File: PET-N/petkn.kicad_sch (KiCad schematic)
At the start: 0 parts

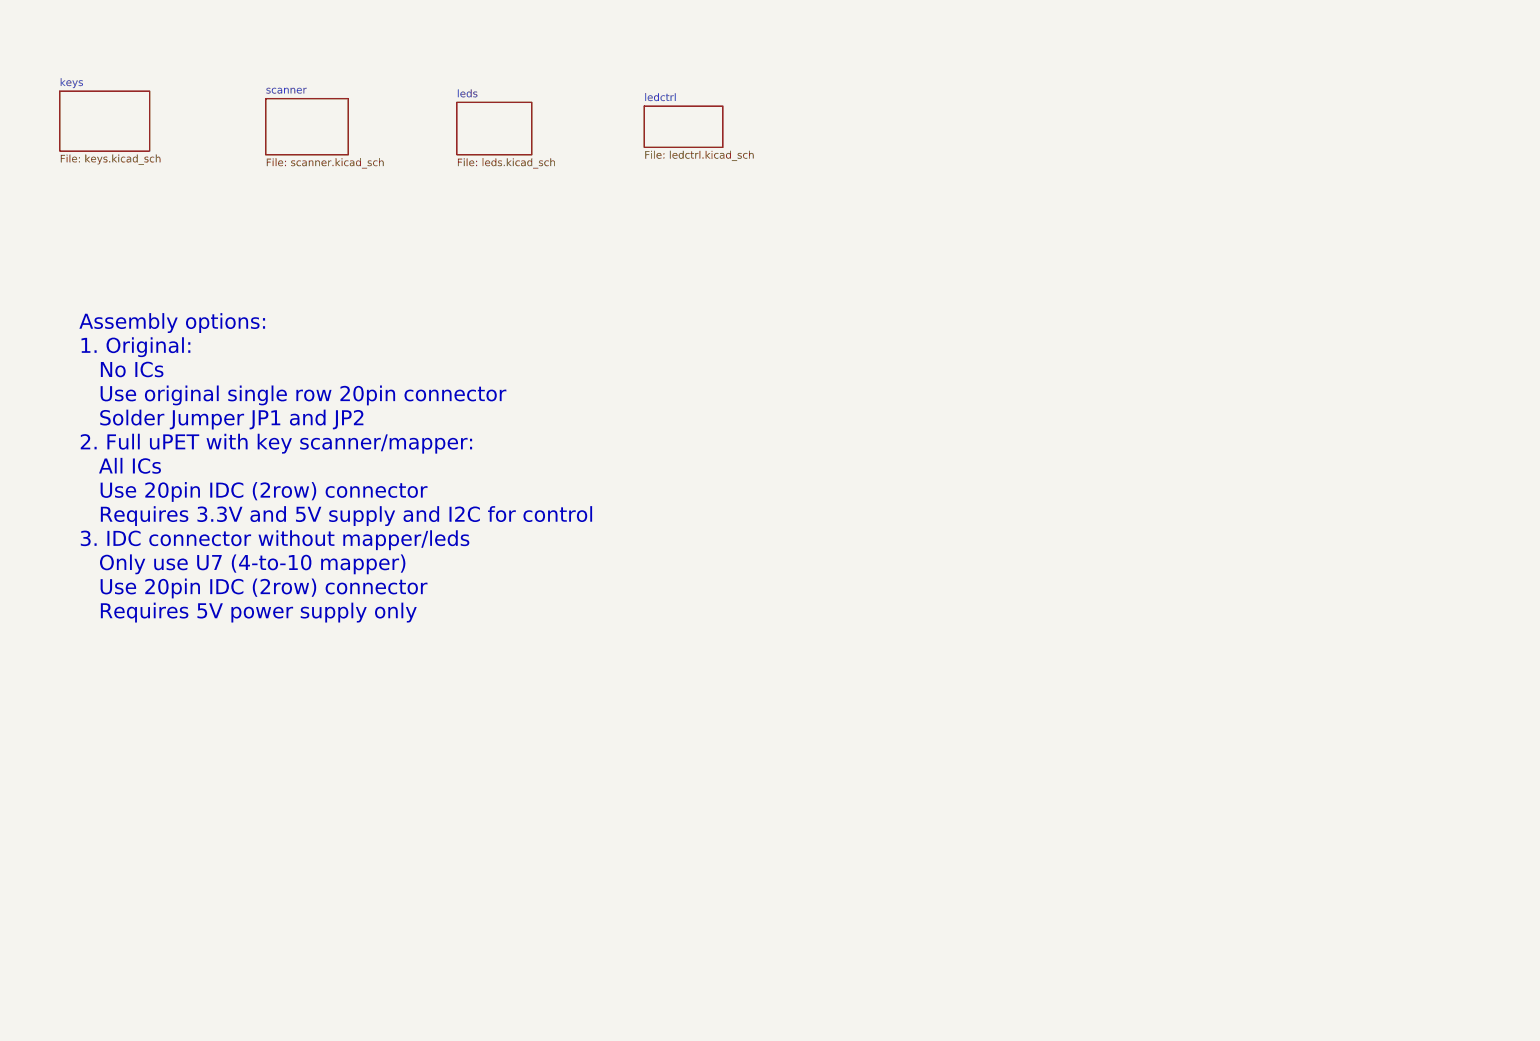
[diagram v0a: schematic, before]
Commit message: almost done routing; last checks still open
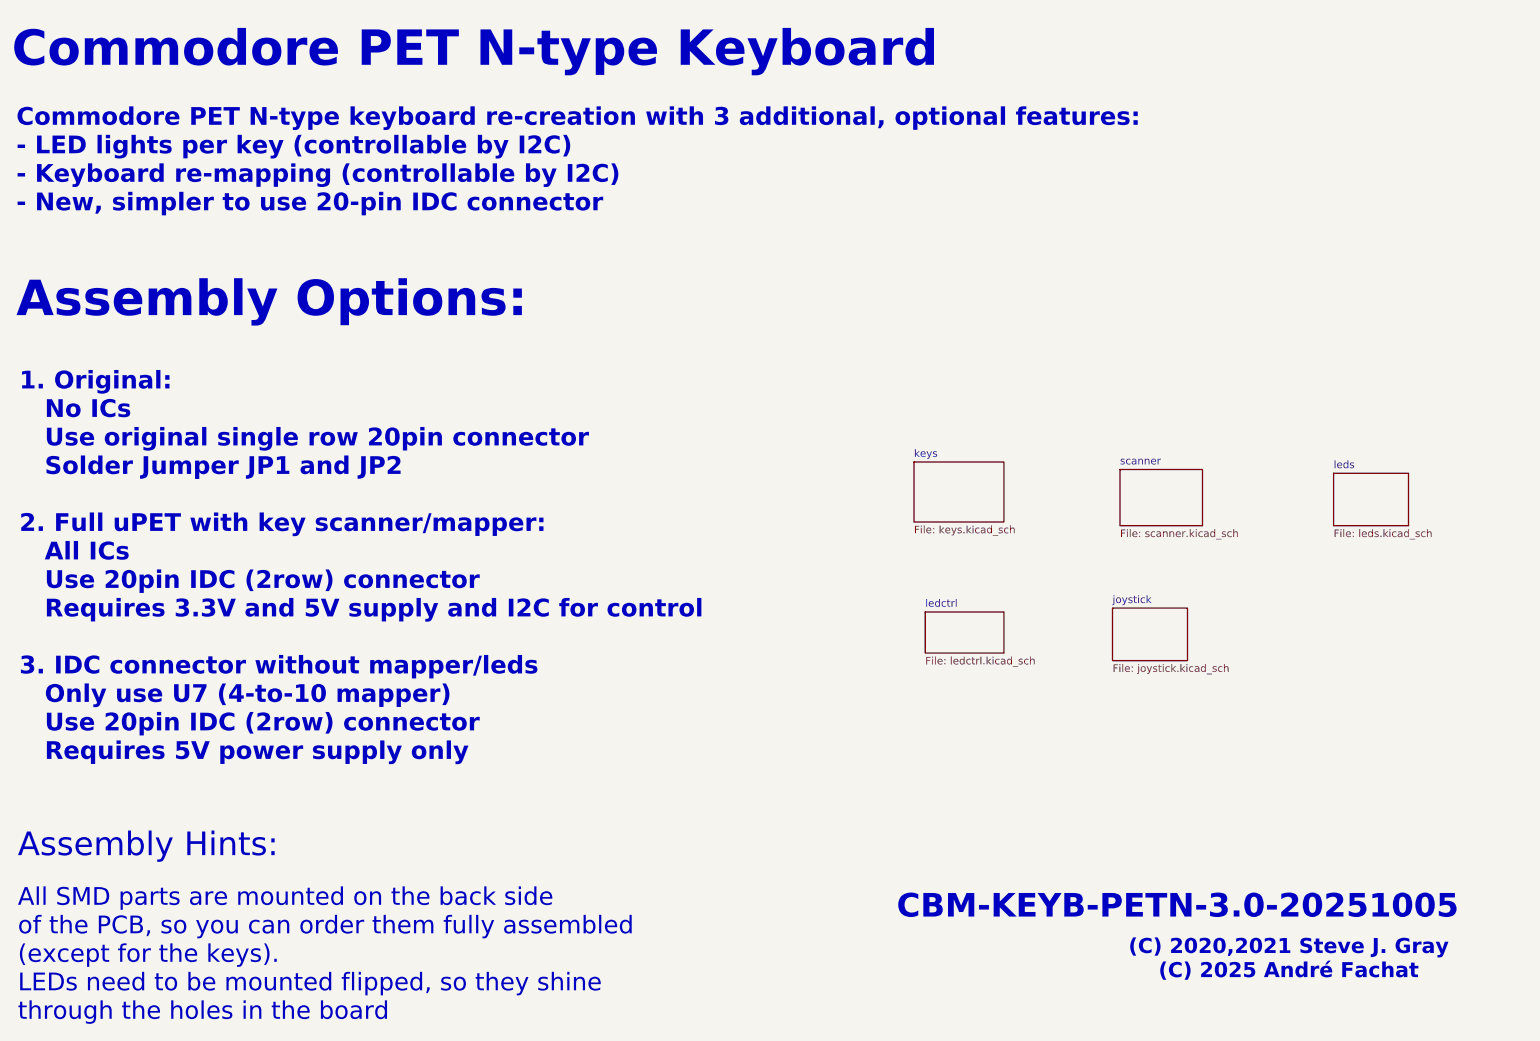
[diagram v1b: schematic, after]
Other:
- added sheet joystick (joystick.kicad_sch)
- note added: "(C) 2020,2021 Steve J. Gray (C) 2025 André Fachat"
- note added: "1. Original: No ICs Use original single row 20pin connector Solder Jumper JP1 and JP2 2. Full uPET with key scanner/mapper: All ICs Use 20pin IDC (2row) connector Requires 3.3V and 5V supply and I2C for control 3. IDC connector without mapper/leds Only use U7 (4-to-10 mapper) Use 20pin IDC (2row) connector Requires 5V power supply only"
- note added: "All SMD parts are mounted on the back side of the PCB, so you can order them fully assembled (except for the keys). LEDs need to be mounted flipped, so they shine through the holes in the board"
- note added: "Assembly Hints:"
- note added: "Assembly Options:"
- note added: "CBM-KEYB-PETN-3.0-20251005"
- note added: "Commodore PET N-type Keyboard"
- note added: "Commodore PET N-type keyboard re-creation with 3 additional, optional features: - LED lights per key (controllable by I2C) - Keyboard re-mapping (controllable by I2C) - New, simpler to use 20-pin IDC connector"
- note removed: "Assembly options: 1. Original: No ICs Use original single row 20pin connector Solder Jumper JP1 and JP2 2. Full uPET with key scanner/mapper: All ICs Use 20pin IDC (2row) connector Requires 3.3V and 5V supply and I2C for control 3. IDC connector without mapper/leds Only use U7 (4-to-10 mapper) Use 20pin IDC (2row) connector Requires 5V power supply only"
- company: Steve J. Gray -> Steve J. Gray, André Fachat
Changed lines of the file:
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@@
 	(title_block
 		(title "PET/CBM \"N\" Keyboard")
-		(date "2020-12-18")
-		(rev "N-V1-R1")
-		(company "Steve J. Gray")
-	)
-	(text "Assembly options:\n1. Original:\n   No ICs\n   Use original single row 20pin connector\n   Solder Jumper JP1 and JP2\n2. Full uPET with key scanner/mapper:\n   All ICs\n   Use 20pin IDC (2row) connector\n   Requires 3.3V and 5V supply and I2C for control\n3. IDC connector without mapper/leds\n   Only use U7 (4-to-10 mapper)\n   Use 20pin IDC (2row) connector\n   Requires 5V power supply only"
-		(exclude_from_sim no)
-		(at 43.942 98.806 0)
+		(date "2025-10-05")
+		(rev "N-V3-R0")
+		(company "Steve J. Gray, André Fachat")
+	)
+	(text "1. Original:\n   No ICs\n   Use original single row 20pin connector\n   Solder Jumper JP1 and JP2\n\n2. Full uPET with key scanner/mapper:\n   All ICs\n   Use 20pin IDC (2row) connector\n   Requires 3.3V and 5V supply and I2C for control\n\n3. IDC connector without mapper/leds\n   Only use U7 (4-to-10 mapper)\n   Use 20pin IDC (2row) connector\n   Requires 5V power supply only"
+		(exclude_from_sim no)
+		(at 33.782 115.57 0)
+		(effects
+			(font
+				(size 3 3)
+				(thickness 0.6)
+				(bold yes)
+			)
+			(justify left)
+		)
+	)
+	(text "All SMD parts are mounted on the back side\nof the PCB, so you can order them fully assembled\n(except for the keys).\nLEDs need to be mounted flipped, so they shine\nthrough the holes in the board"
+		(exclude_from_sim no)
+		(at 33.528 181.356 0)
+		(effects
+			(font
+				(size 3 3)
+				(thickness 0.375)
+			)
+			(justify left)
+		)
+	)
+	(text "Commodore PET N-type keyboard re-creation with 3 additional, optional features:\n- LED lights per key (controllable by I2C)\n- Keyboard re-mapping (controllable by I2C)\n- New, simpler to use 20-pin IDC connector"
+		(exclude_from_sim no)
+		(at 33.274 46.736 0)
+		(effects
+			(font
+				(size 3 3)
+				(thickness 0.6)
+				(bold yes)
+			)
+			(justify left)
+		)
+	)
+	(text "Assembly Options:"
+		(exclude_from_sim no)
+		(at 33.274 70.358 0)
+		(effects
+			(font
+				(size 6 6)
+				(thickness 1.2)
+				(bold yes)
+			)
+			(justify left)
+		)
+	)
+	(text "(C) 2020,2021 Steve J. Gray\n(C) 2025 André Fachat"
+		(exclude_from_sim no)
+		(at 248.92 182.118 0)
 		(effects
 			(font
 				(size 2.54 2.54)
-			)
-			(justify left)
-		)
-	)
-	(sheet
-		(at 40.64 34.925)
+				(thickness 0.508)
+				(bold yes)
+			)
+		)
+	)
+	(text "Assembly Hints:"
+		(exclude_from_sim no)
+		(at 33.528 162.814 0)
+		(effects
+			(font
+				(size 4 4)
+				(thickness 0.75)
+			)
+			(justify left)
+		)
+	)
+	(text "Commodore PET N-type Keyboard"
+		(exclude_from_sim no)
+		(at 32.512 27.94 0)
+		(effects
+			(font
+				(size 6 6)
+				(thickness 1.2)
+				(bold yes)
+			)
+			(justify left)
+		)
+	)
+	(text "CBM-KEYB-PETN-3.0-20251005"
+		(exclude_from_sim no)
+		(at 230.124 173.228 0)
+		(effects
+			(font
+				(size 4 4)
+				(thickness 0.9)
+				(bold yes)
+			)
+		)
+	)
+	(sheet
+		(at 185.42 97.79)
 		(size 15.24 10.16)
 		(exclude_from_sim no)
@@
 		)
 		(property "Sheetname" "keys"
-			(at 40.64 34.2134 0)
+			(at 185.42 97.0784 0)
 			(effects
 				(font
@@
 		)
 		(property "Sheetfile" "keys.kicad_sch"
-			(at 40.64 45.6696 0)
+			(at 185.42 108.5346 0)
 			(effects
 				(font
@@
 	)
 	(sheet
-		(at 75.565 36.195)
+		(at 220.345 99.06)
 		(size 13.97 9.525)
 		(exclude_from_sim no)
@@
 		)
 		(property "Sheetname" "scanner"
-			(at 75.565 35.4834 0)
+			(at 220.345 98.3484 0)
 			(effects
 				(font
@@
 		)
 		(property "Sheetfile" "scanner.kicad_sch"
-			(at 75.565 46.3046 0)
+			(at 220.345 109.1696 0)
 			(effects
 				(font
@@
 	)
 	(sheet
-		(at 107.95 36.83)
+		(at 219.075 122.555)
 		(size 12.7 8.89)
 		(exclude_from_sim no)
@@
 			(color 0 0 0 0.0000)
 		)
+		(property "Sheetname" "joystick"
+			(at 219.075 121.8434 0)
+			(effects
+				(font
+					(size 1.27 1.27)
+				)
+				(justify left bottom)
+			)
+		)
+		(property "Sheetfile" "joystick.kicad_sch"
+			(at 219.075 132.0296 0)
+			(effects
+				(font
+					(size 1.27 1.27)
+				)
+				(justify left top)
+			)
+		)
+		(instances
+			(project "petkn"
+				(path "/a0727808-af70-4056-b2ee-ab828c2acfbd"
+					(page "6")
+				)
+			)
+		)
+	)
+	(sheet
+		(at 256.54 99.695)
+		(size 12.7 8.89)
+		(exclude_from_sim no)
+		(in_bom yes)
+		(on_board yes)
+		(dnp no)
+		(fields_autoplaced yes)
+		(stroke
+			(width 0.1524)
+			(type solid)
+		)
+		(fill
+			(color 0 0 0 0.0000)
+		)
 		(property "Sheetname" "leds"
-			(at 107.95 36.1184 0)
+			(at 256.54 98.9834 0)
 			(effects
 				(font
@@
 		)
 		(property "Sheetfile" "leds.kicad_sch"
-			(at 107.95 46.3046 0)
+			(at 256.54 109.1696 0)
 			(effects
 				(font
@@
 	)
 	(sheet
-		(at 139.7 37.465)
+		(at 187.325 123.19)
 		(size 13.335 6.985)
 		(exclude_from_sim no)
@@
 		)
 		(property "Sheetname" "ledctrl"
-			(at 139.7 36.7534 0)
+			(at 187.325 122.4784 0)
 			(effects
 				(font
@@
 		)
 		(property "Sheetfile" "ledctrl.kicad_sch"
-			(at 139.7 45.0346 0)
-			(effects
-				(font
+			(at 187.325 130.7596 0)
+			(effects
+				(font

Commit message: hopefully final schem and layout for 3.0A
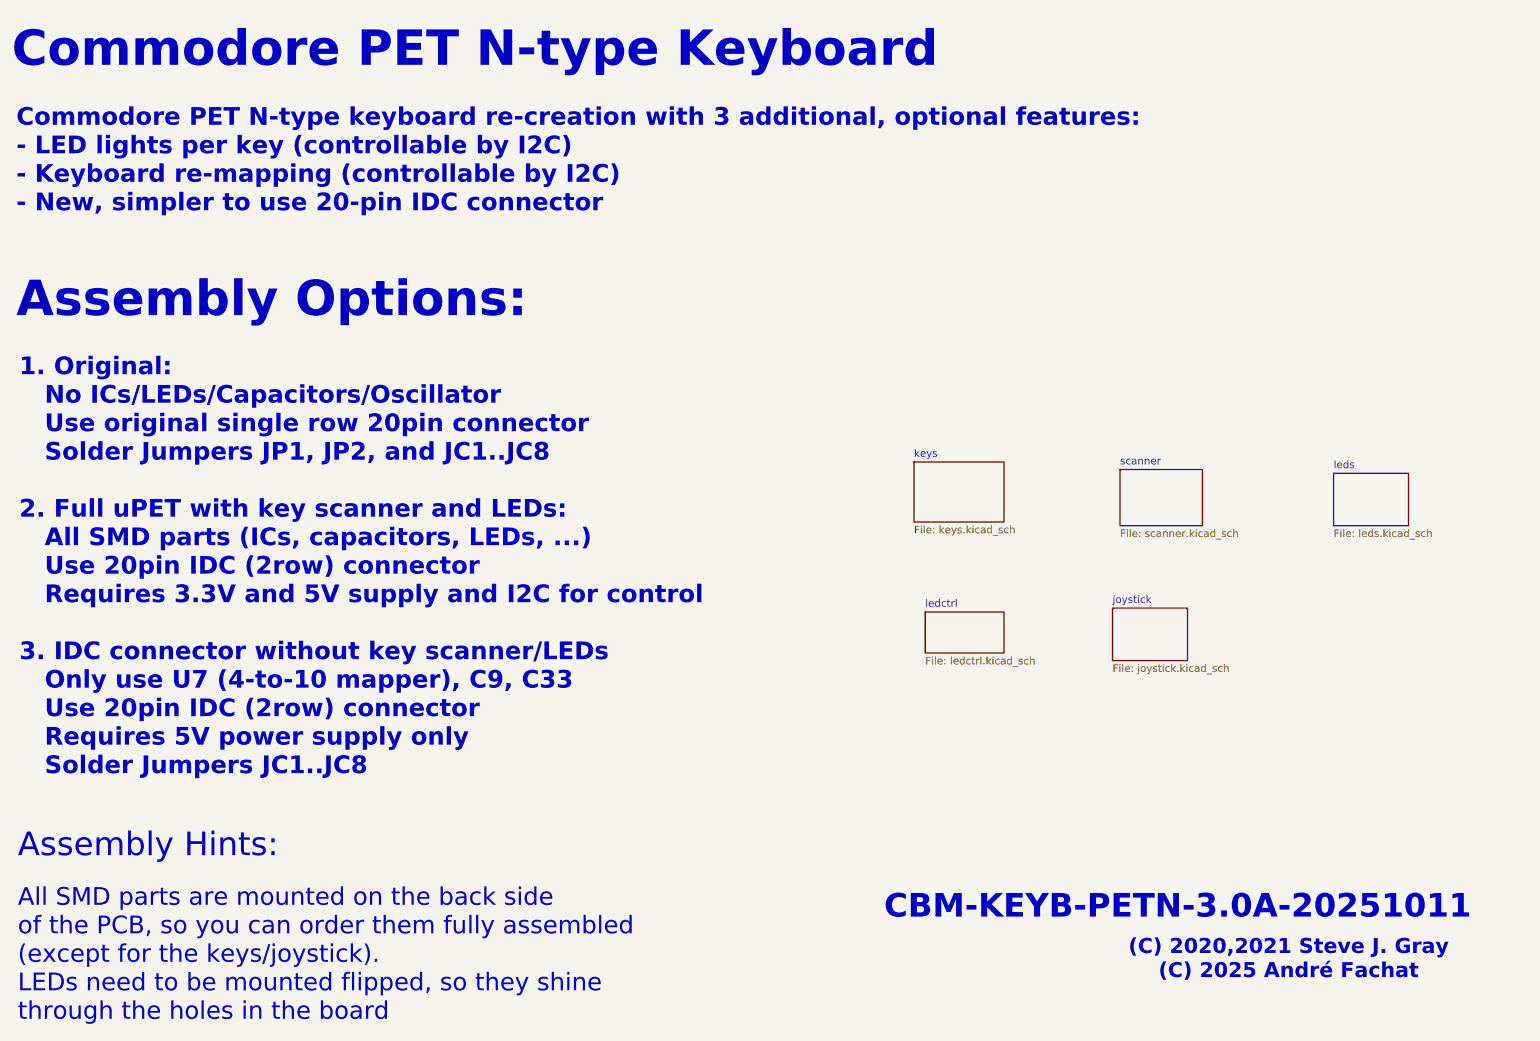
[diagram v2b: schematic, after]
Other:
- note added: "1. Original: No ICs/LEDs/Capacitors/Oscillator Use original single row 20pin connector Solder Jumpers JP1, JP2, and JC1..JC8 2. Full uPET with key scanner and LEDs: All SMD parts (ICs, capacitors, LEDs, ...) Use 20pin IDC (2row) connector Requires 3.3V and 5V supply and I2C for control 3. IDC connector without key scanner/LEDs Only use U7 (4-to-10 mapper), C9, C33 Use 20pin IDC (2row) connector R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"
- note added: "All SMD parts are mounted on the back side of the PCB, so you can order them fully assembled (except for the keys/joystick). LEDs need to be mounted flipped, so they shine through the holes in the board"
- note added: "CBM-KEYB-PETN-3.0A-20251011"
- note removed: "1. Original: No ICs Use original single row 20pin connector Solder Jumper JP1 and JP2 2. Full uPET with key scanner/mapper: All ICs Use 20pin IDC (2row) connector Requires 3.3V and 5V supply and I2C for control 3. IDC connector without mapper/leds Only use U7 (4-to-10 mapper) Use 20pin IDC (2row) connector Requires 5V power supply only"
- note removed: "All SMD parts are mounted on the back side of the PCB, so you can order them fully assembled (except for the keys). LEDs need to be mounted flipped, so they shine through the holes in the board"
- note removed: "CBM-KEYB-PETN-3.0-20251005"
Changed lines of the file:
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@@
 		(company "Steve J. Gray, André Fachat")
 	)
-	(text "1. Original:\n   No ICs\n   Use original single row 20pin connector\n   Solder Jumper JP1 and JP2\n\n2. Full uPET with key scanner/mapper:\n   All ICs\n   Use 20pin IDC (2row) connector\n   Requires 3.3V and 5V supply and I2C for control\n\n3. IDC connector without mapper/leds\n   Only use U7 (4-to-10 mapper)\n   Use 20pin IDC (2row) connector\n   Requires 5V power supply only"
+	(text "1. Original:\n   No ICs/LEDs/Capacitors/Oscillator\n   Use original single row 20pin connector\n   Solder Jumpers JP1, JP2, and JC1..JC8\n\n2. Full uPET with key scanner and LEDs:\n   All SMD parts (ICs, capacitors, LEDs, ...)\n   Use 20pin IDC (2row) connector\n   Requires 3.3V and 5V supply and I2C for control\n\n3. IDC connector without key scanner/LEDs\n   Only use U7 (4-to-10 mapper), C9, C33\n   Use 20pin IDC (2row) connector\n   Requires 5V power supply only\n   Solder Jumpers JC1..JC8"
 		(exclude_from_sim no)
 		(at 33.782 115.57 0)
@@
 		)
 	)
-	(text "All SMD parts are mounted on the back side\nof the PCB, so you can order them fully assembled\n(except for the keys).\nLEDs need to be mounted flipped, so they shine\nthrough the holes in the board"
+	(text "All SMD parts are mounted on the back side\nof the PCB, so you can order them fully assembled\n(except for the keys/joystick).\nLEDs need to be mounted flipped, so they shine\nthrough the holes in the board"
 		(exclude_from_sim no)
 		(at 33.528 181.356 0)
@@
 		)
 	)
-	(text "CBM-KEYB-PETN-3.0-20251005"
+	(text "CBM-KEYB-PETN-3.0A-20251011"
 		(exclude_from_sim no)
 		(at 230.124 173.228 0)
